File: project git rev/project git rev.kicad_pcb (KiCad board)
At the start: 2 copper layers, 94 x 44 mm, 31 parts, among them J1 Conn_01x03, J11 Conn_01x02, J4 Conn_01x02, J7 Conn_01x02, U1 LM358

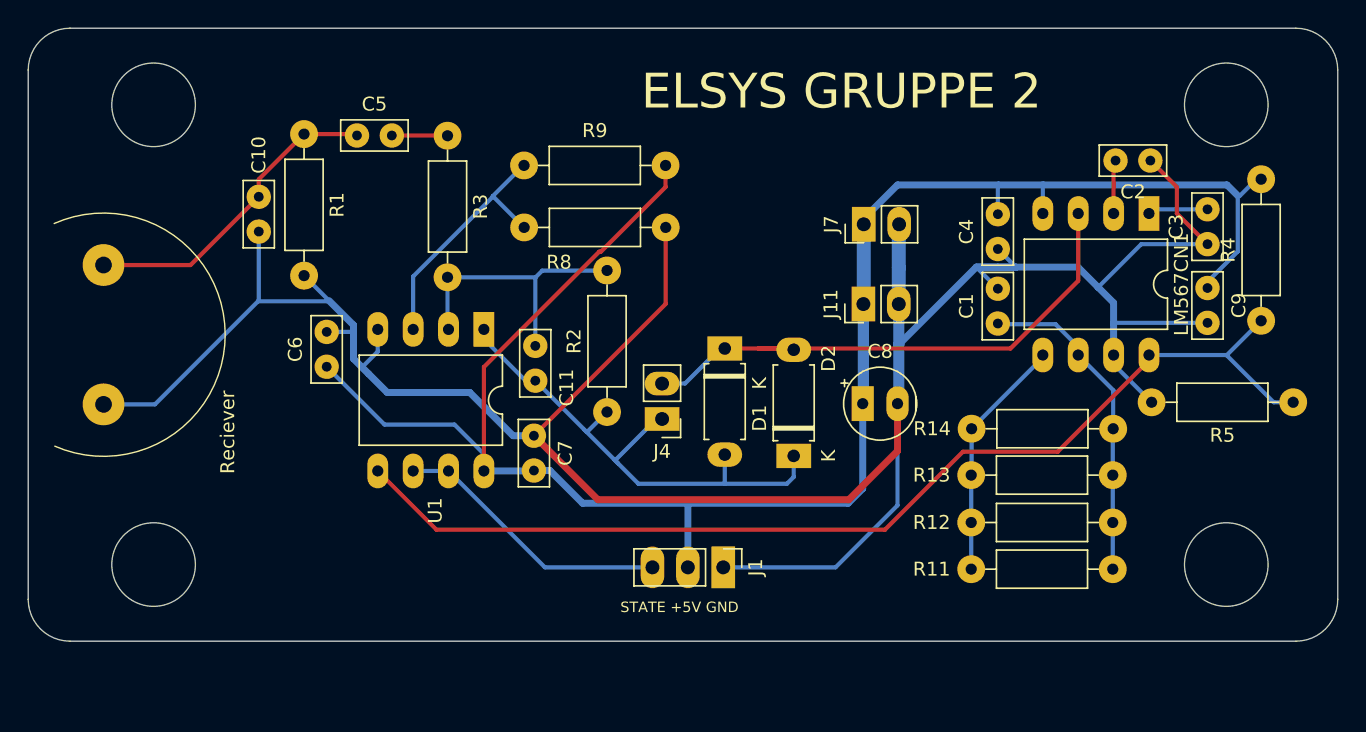
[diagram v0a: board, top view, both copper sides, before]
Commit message: La til MCP adcen i kretsen og bestilte 👍
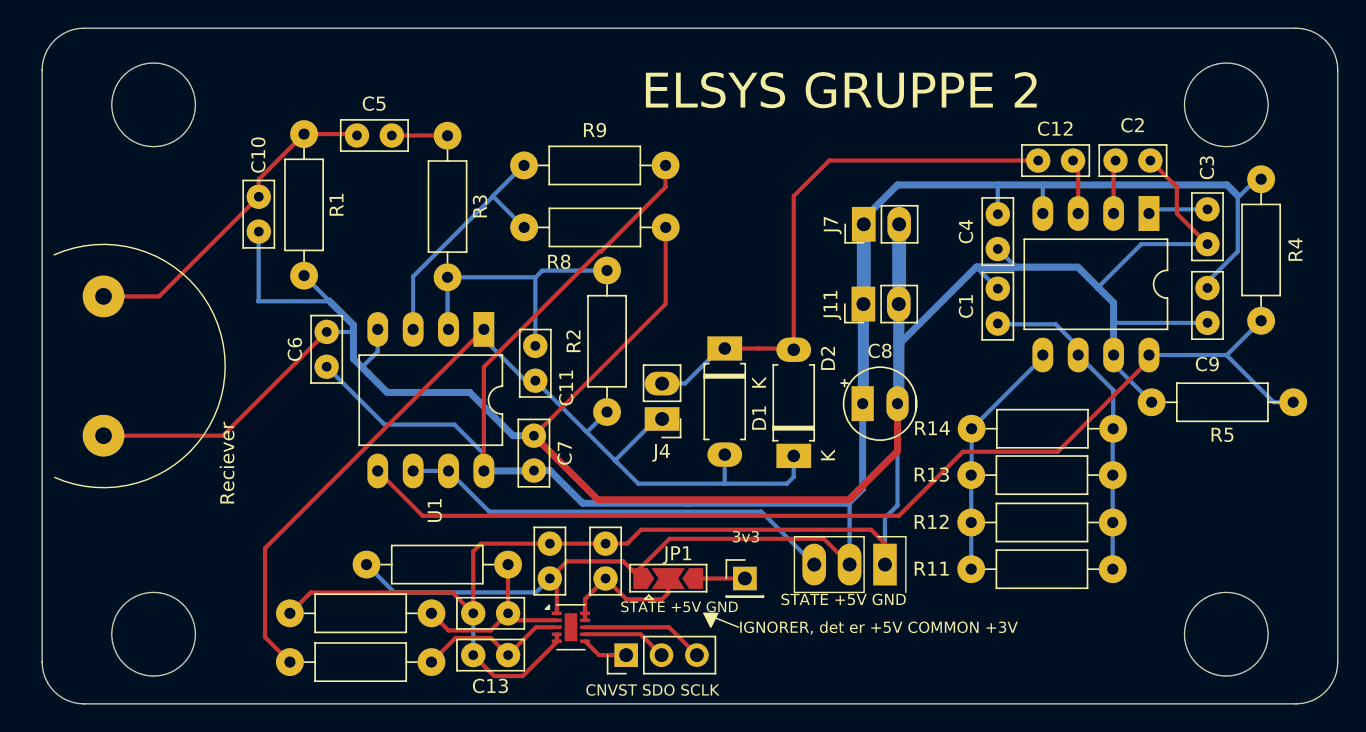
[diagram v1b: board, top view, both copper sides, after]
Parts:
- added C12: 10n, UR:C_Rect_L4.6mm_W2.0mm_P2.50mm_MKS02_FKP02, F.Cu at (182.5, 86.0)
- added C13: C, UR:C_Rect_L4.6mm_W2.0mm_P2.50mm_MKS02_FKP02, F.Cu at (144.4, 121.5)
- added C14: 100n, UR:C_Rect_L4.6mm_W2.0mm_P2.50mm_MKS02_FKP02, F.Cu at (151.4, 116.0)
- added C15: 1u, UR:C_Rect_L4.6mm_W2.0mm_P2.50mm_MKS02_FKP02, F.Cu at (141.9, 118.5)
- added C16: 10u, UR:C_Rect_L4.6mm_W2.0mm_P2.50mm_MKS02_FKP02, F.Cu at (147.4, 116.0)
- added J2: Conn_01x03_Pin, Connector_PinHeader_2.54mm:PinHeader_1x03_P2.54mm_Vertical, F.Cu at (152.9, 121.5)
- added J3: 3.3V input, Connector_PinHeader_2.54mm:PinHeader_1x01_P2.54mm_Vertical, F.Cu at (161.4, 116.0)
- added JP1: SolderJumper_3_Open, Jumper:SolderJumper-3_P2.0mm_Open_TrianglePad1.0x1.5mm, F.Cu at (155.9, 116.0)
- added R10: 5625, UR:R_Axial_DIN0207_L6.3mm_D2.5mm_P10.16mm_Horizontal, F.Cu at (138.9, 118.5)
- added R6: R, UR:R_Axial_DIN0207_L6.3mm_D2.5mm_P10.16mm_Horizontal, F.Cu at (128.8, 122.0)
- added R7: 10k, UR:R_Axial_DIN0207_L6.3mm_D2.5mm_P10.16mm_Horizontal, F.Cu at (144.4, 115.0)
- added U2: ~, Package_DFN_QFN:TDFN-10-1EP_2x3mm_P0.5mm_EP0.9x2mm, F.Cu at (149.0, 119.5)
- moved J1 11.6 mm to (171.5, 115.0)
- moved MK1 2.25 mm to (115.4, 105.8)
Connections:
- net Net-(D1-A) renamed MIC
- LM567CN1 pad 3: Signal -> Net-(LM567CN1-Signal)
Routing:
- net GND: track 198.4 -> 255.7 mm
- net +5V: track 137.3 -> 179.2 mm
- net MIC: track 38.0 -> 69.2 mm
- net Net-(U2-AVdd): track 0.00 -> 13.7 mm
- net State: track 20.0 -> 31.6 mm
- net Net-(U2-Ain+): track 0.00 -> 10.8 mm
- net Net-(JP1-C): track 0.00 -> 9.97 mm
- net Net-(J2-Pin_3): track 0.00 -> 8.86 mm
- net Net-(J2-Pin_2): track 0.00 -> 6.11 mm
- net Net-(LM567CN1-Signal): track 0.00 -> 5.38 mm
- net Net-(J3-Pin_1): track 0.00 -> 3.50 mm
- net Net-(J2-Pin_1): track 0.00 -> 3.36 mm
- net Net-(MK1-+): track 23.2 -> 24.1 mm
- net Net-(LM567CN1-Output): track 79.1 -> 78.3 mm
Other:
- board size 94 x 44 mm -> 93 x 48.5 mm
- board text added: "3v3"
- board text added: "CNVST SDO SCLK"
- board text added: "IGNORER, det er +5V COMMON +3V"
